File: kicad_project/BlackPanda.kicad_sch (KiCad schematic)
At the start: 91 parts, among them J1 Conn_01x04_Female, J2 USB_A TE Connectivity 292303-7, P1 USB-C-USB-3.2-rescue_USB_C_Pl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, Q1 DDTA143ECA-7-F P08, Q2 DDTA143ECA-7-F P08, Q3 PDTC114EU, SW1 SW_Push, U1 SIS427EDN-T1-GE3, U10 TJA1042TK-3, U11 TJA1042TK-3, U12 XL1509-3.3, U2 SiP32431DR3, U4 NEO-M8M, U5 TPS54560BDDA, U6 TPS2549IRTETQ1, U7 STM32F413RGTx, U8 TJA1042TK-3, U9 TJA1042TK-3, Y1 X322516MLB4SI

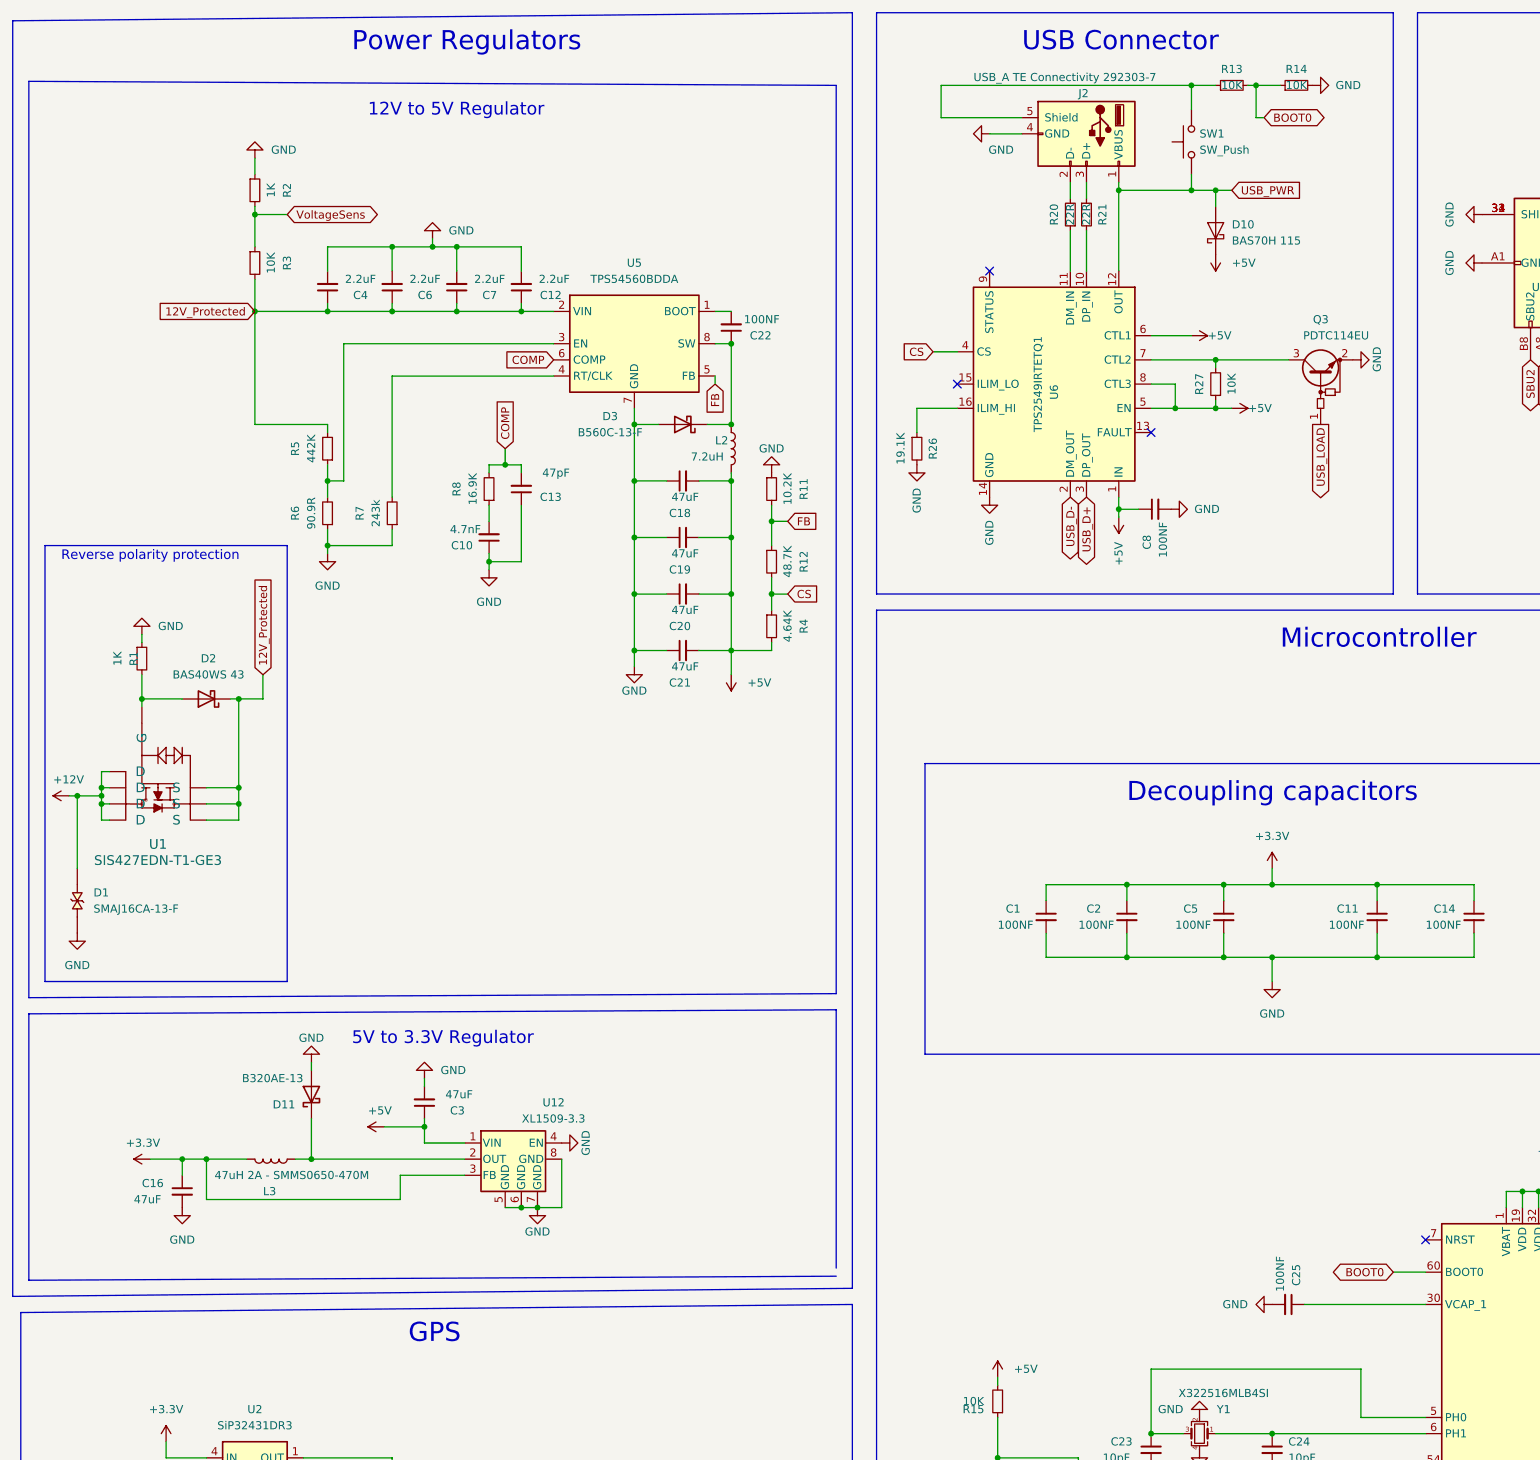
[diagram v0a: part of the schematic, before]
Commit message: -
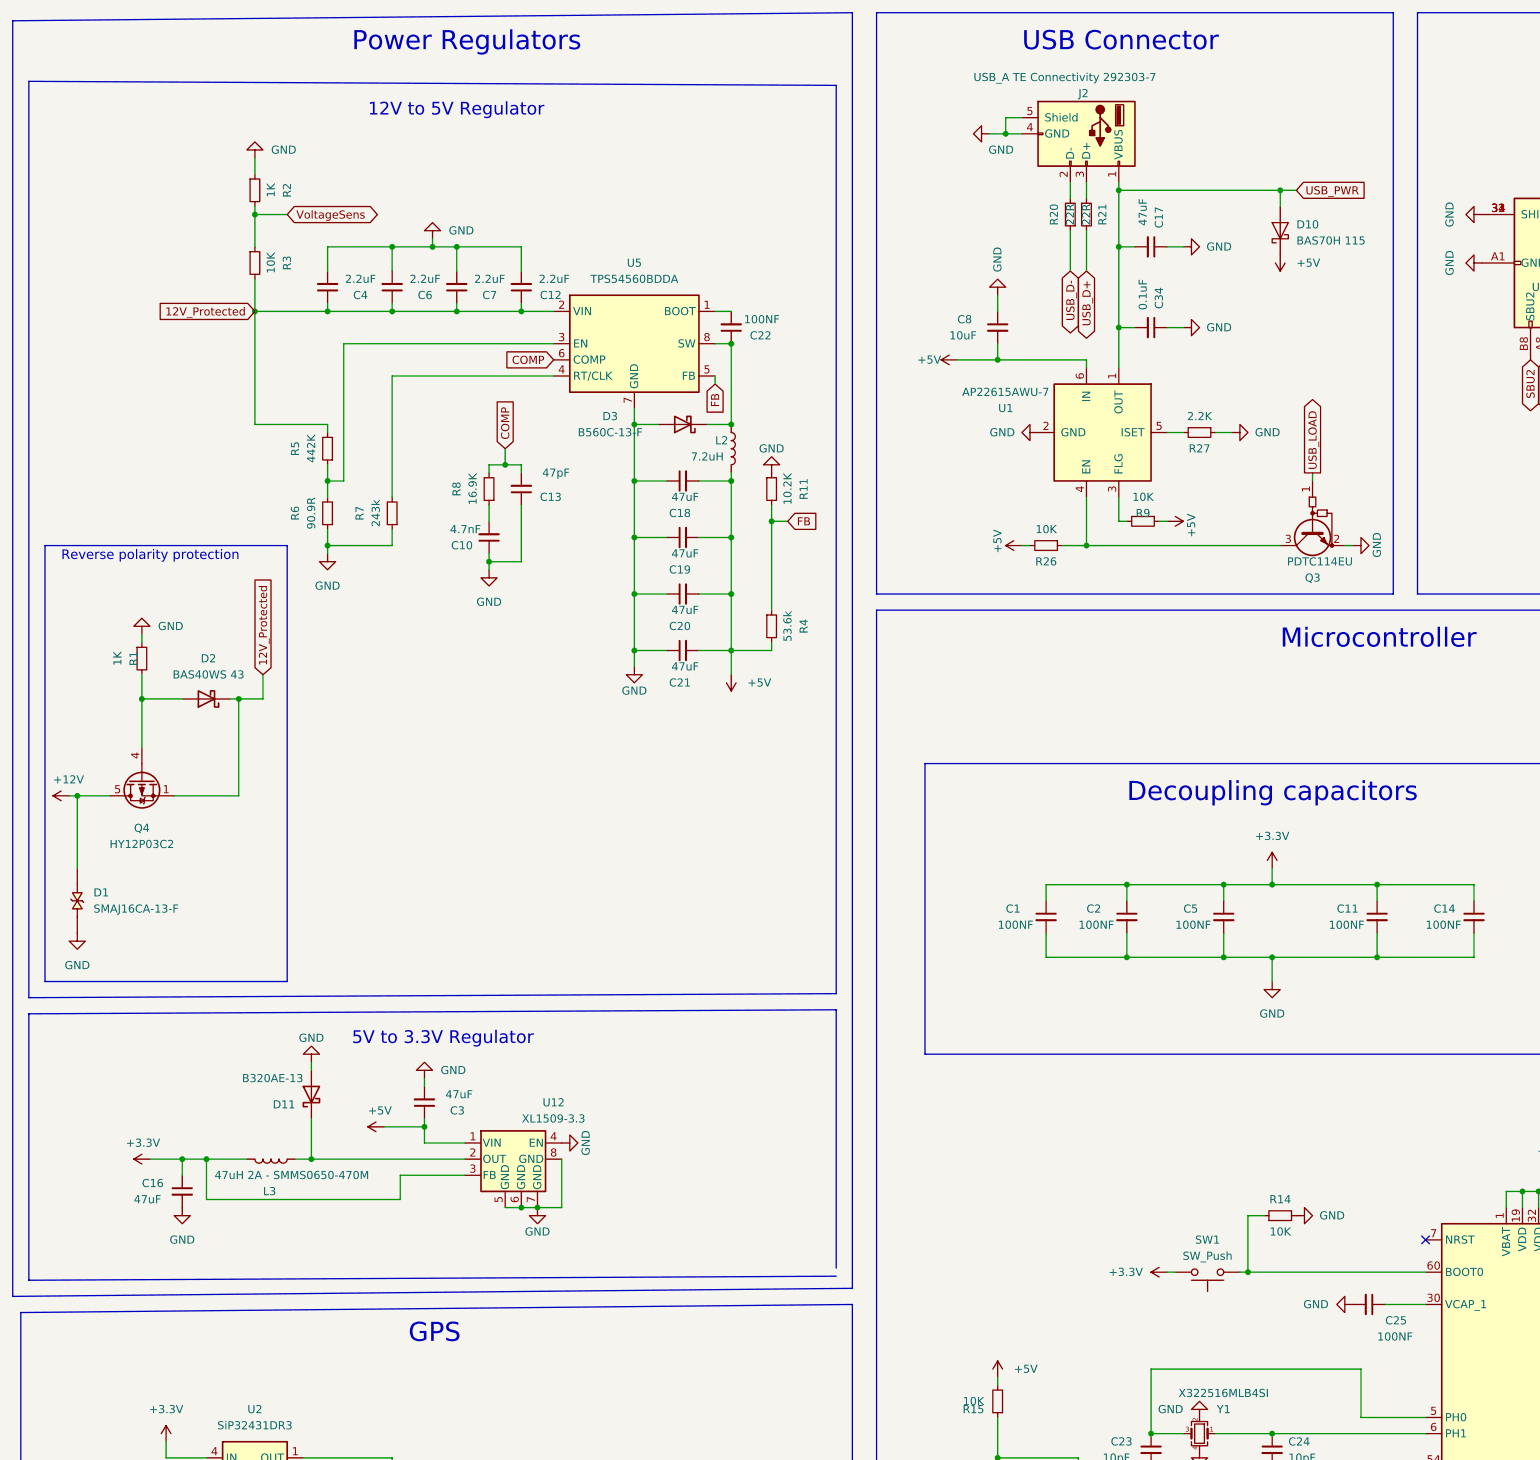
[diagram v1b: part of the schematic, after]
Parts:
- removed R12: 48.7K, Resistor_SMD:R_0603_1608Metric, symbol Device:R_Small
- removed R13: 10K, Resistor_SMD:R_0402_1005Metric, symbol Device:R_Small
- removed U1: SIS427EDN-T1-GE3, BlackPanda:SIS427EDN-T1-GE3, symbol SIS427EDN-T1-GE3:SIS427EDN-T1-GE3
- removed U6: TPS2549IRTETQ1, Package_DFN_QFN:WQFN-16-1EP_3x3mm_P0.5mm_EP1.75x1.75mm, symbol Interface_USB:TPS2549IRTETQ1
- added C17: 47uF, Capacitor_SMD:C_0805_2012Metric, symbol Device:C_Small
- added C34: 0.1uF, Capacitor_SMD:C_0402_1005Metric, symbol Device:C_Small
- added Q4: HY12P03C2, Package_SO:PowerPAK_SO-8_Single, symbol Transistor_FET:Si7141DP
- added R9: 10K, Resistor_SMD:R_0402_1005Metric, symbol Device:R_Small
- added U1: AP22615AWU-7, Package_TO_SOT_SMD:SOT-23-6, symbol Analog_ADC:AP22615AWU-7
- C8: value 100NF -> 10uF
- R26: value 19.1K -> 10K
- R27: value 10K -> 2.2K
- R4: value 4.64K -> 53.6k
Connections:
- net CS is gone; now on net FB: R4.1
- net +12V: now also Q4.5 (D)
- net +3V3: now also SW1.2
- net +5V: now also C8.2, R26.2, R9.1, U1.6 (IN); no longer C8.1, R27.1
- net 12V_Protected: now also Q4.1 (S), Q4.2 (S), Q4.3 (S)
- net GND: now also C8.1, J2.5 (Shield), R27.1, C17.1, C34.1, U1.2 (GND); no longer C8.2, R26.2
- net USB_D+: now also R21.2
- net USB_D-: now also R20.1
- net USB_PWR: now also C17.2, C34.2, U1.1 (OUT); no longer SW1.1
- net at D2.2 (A), R1.2: now also Q4.4 (G)
- net at R26.1: now also Q3.3 (C), U1.4 (EN)
- net at R27.2: now also U1.5 (ISET); no longer Q3.3 (C)
- net BOOT0: no longer names the net of R14.1, U7.60 (BOOT0)
- net BOOT0: now also SW1.1
- new net: R9.2, U1.3 (FLG)
- no-connect marks 25 -> 22
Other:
- moved on the sheet: C25, C8, D10, Q3, R14, R26, R27, SW1
